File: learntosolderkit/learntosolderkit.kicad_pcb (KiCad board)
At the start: 2 copper layers, 58 x 34.5 mm, 11 parts, among them SW1 SW_Push, SW2 SW_Push, SW3 SW_Push, U1 NE555P

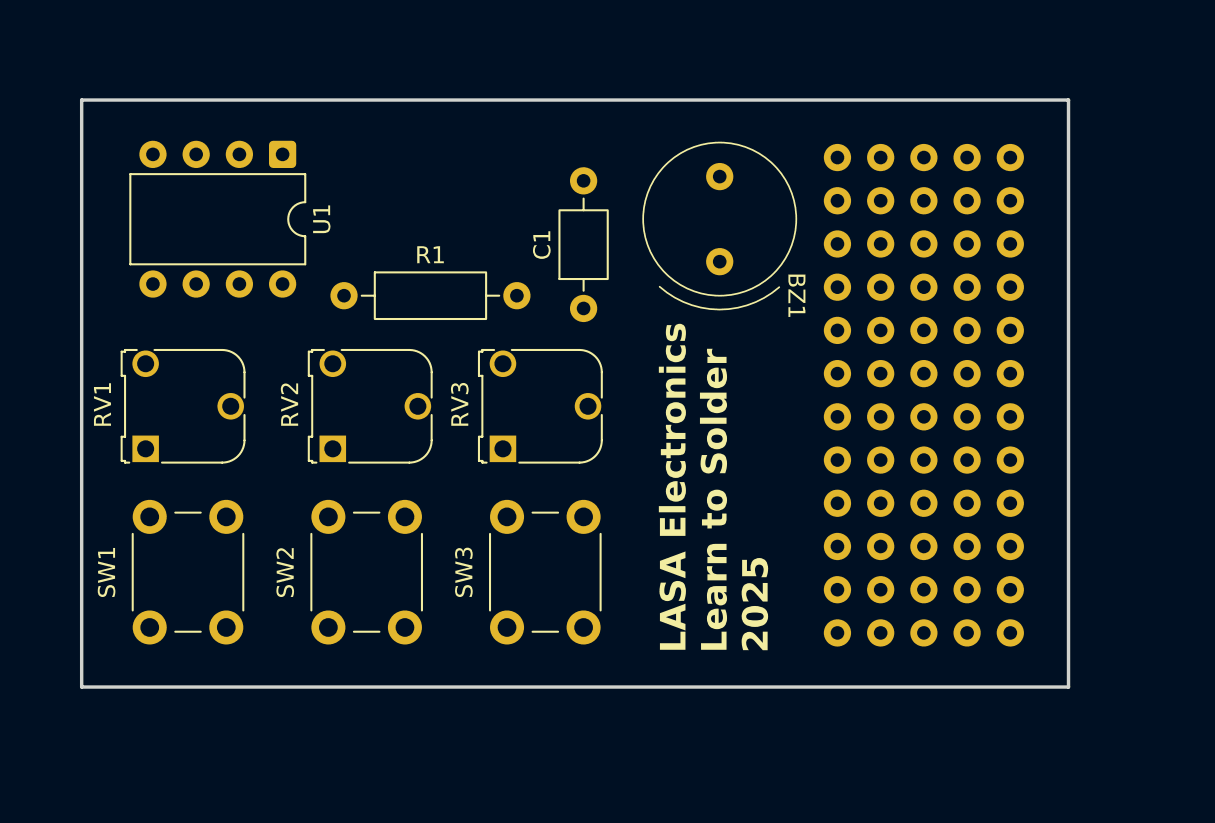
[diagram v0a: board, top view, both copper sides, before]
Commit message: Finish up
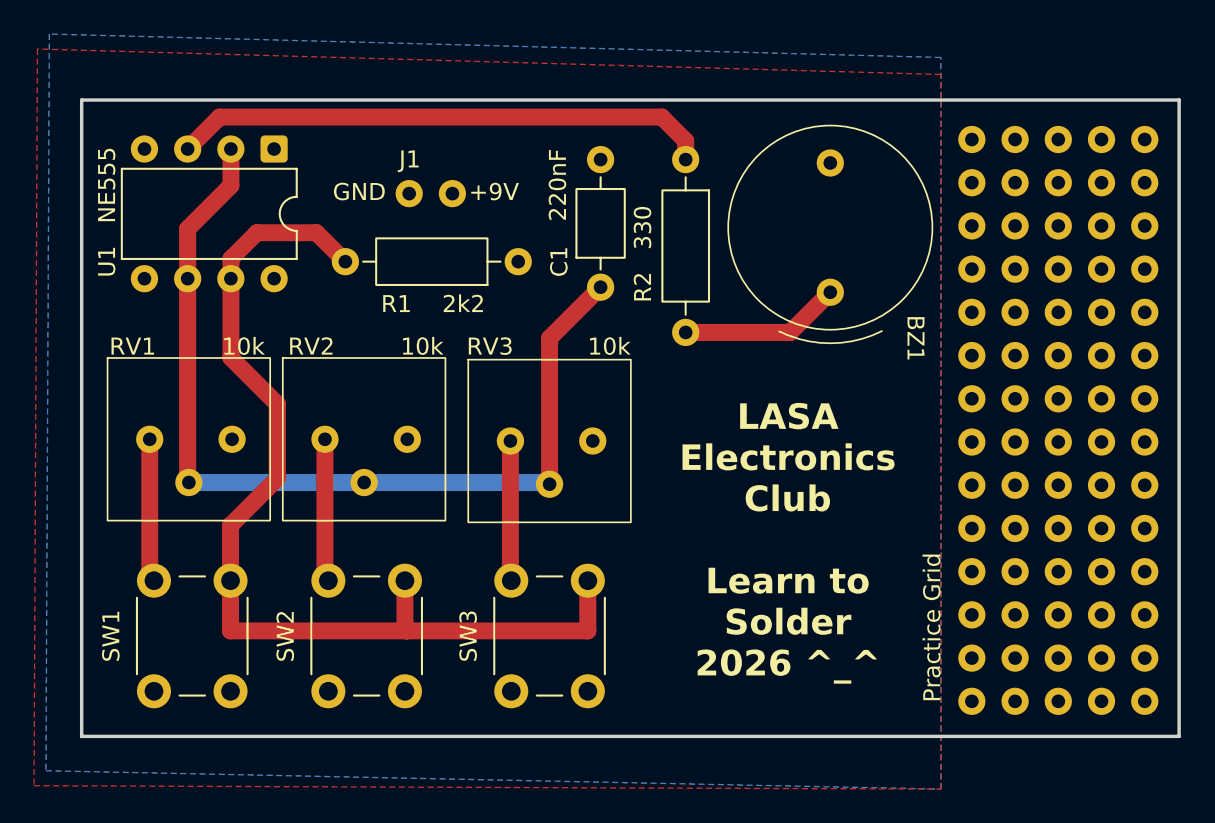
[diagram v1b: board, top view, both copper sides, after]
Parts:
- added J1: 9V Connector, 1_my_custom_library:9v_dc_batt_2_pin, F.Cu at (129.8, 77.0)
- added R2: 330, Resistor_THT:R_Axial_DIN0207_L6.3mm_D2.5mm_P10.16mm_Horizontal, F.Cu at (146.0, 75.0)
- BZ1: value HNB-09A05 self drive -> 42R Passive Buzzer
- C1: value 100n -> 220n
- RV1, RV2, RV3: footprint Potentiometer_THT:Potentiometer_Runtron_RM-065_Vertical -> 1_my_custom_library:3386P_Trimmer
- moved R1 10.4 mm to (136.2, 81.0), turned to 180 degrees
- moved REF** 7.97 mm to (170.4, 76.4)
- moved BZ1 6.52 mm to (154.5, 79.0)
- moved SW1 3.76 mm to (119.2, 99.8)
- moved SW3 3.76 mm to (140.2, 99.8)
- moved SW2 3.75 mm to (129.5, 99.8)
- moved RV3 2.78 mm to (138.0, 91.5), turned to 0 degrees
- moved RV1 2.60 mm to (116.8, 91.4), turned to 0 degrees
- moved RV2 1.92 mm to (127.1, 91.4), turned to 0 degrees
- moved C1 1.60 mm to (141.0, 82.5)
- moved U1 0.59 mm to (121.8, 74.4)
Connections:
- net +5V renamed +9V
- BZ1 pad 1: buzz -> Net-(BZ1-+)
- RV1 pad 1: Net-(RV1-Pad1) -> unconnected-(RV1-Pad1)
- RV1 pad 2: unconnected-(RV1-Pad2) -> Net-(U1-THR)
- RV1 pad 3: Net-(U1-THR) -> Net-(RV1-Pad3)
- RV2 pad 1: Net-(RV2-Pad1) -> unconnected-(RV2-Pad1)
- RV2 pad 2: unconnected-(RV2-Pad2) -> Net-(U1-THR)
- RV2 pad 3: Net-(U1-THR) -> Net-(RV2-Pad3)
- RV3 pad 1: Net-(RV3-Pad1) -> unconnected-(RV3-Pad1)
- RV3 pad 2: unconnected-(RV3-Pad2) -> Net-(U1-THR)
- RV3 pad 3: Net-(U1-THR) -> Net-(RV3-Pad3)
- SW1 pad 2: Net-(RV1-Pad1) -> Net-(RV1-Pad3)
- SW2 pad 2: Net-(RV2-Pad1) -> Net-(RV2-Pad3)
- SW3 pad 2: Net-(RV3-Pad1) -> Net-(RV3-Pad3)
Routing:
- net Net-(U1-DIS): track 0.00 -> 59.2 mm
- net Net-(U1-THR): track 0.00 -> 55.0 mm
- net buzz: track 0.00 -> 31.7 mm
- net Net-(BZ1-+): track 0.00 -> 9.48 mm
- net Net-(RV1-Pad3): track 0.00 -> 8.41 mm
- net Net-(RV2-Pad3): track 0.00 -> 8.39 mm
- net Net-(RV3-Pad3): track 0.00 -> 8.23 mm
- added copper zone on B.Cu, net +9V
- added copper zone on F.Cu, net GND
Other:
- board size 58 x 34.5 mm -> 64.5 x 37.4 mm
- board text added: "10k"
- board text added: "220nF"
- board text added: "2k2"
- board text added: "330"
- board text added: "LASA Electronics Club Learn to Solder 2026 ^_^"
- board text added: "NE555"
- board text added: "Practice Grid"
- board text removed: "LASA Electronics Learn to Solder 2025"
